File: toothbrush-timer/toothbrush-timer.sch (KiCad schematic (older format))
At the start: 19 parts, among them Q1 IRL2244, Q2 IRL6244, SW1 Power, U1 Arduino_Pro_Mini

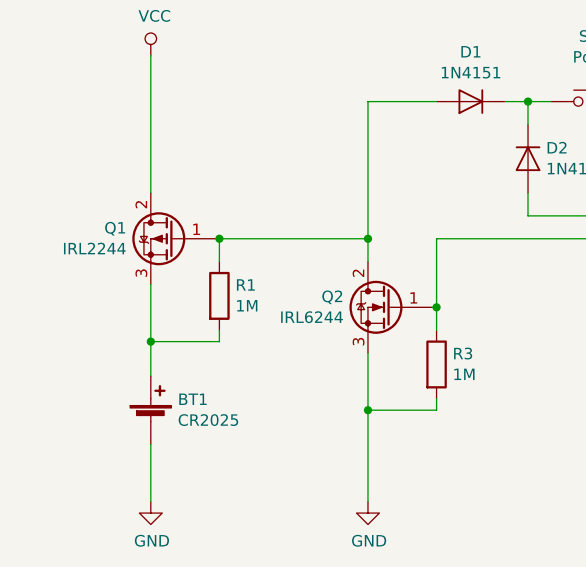
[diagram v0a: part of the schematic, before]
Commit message: Updated toohtbrush-timer
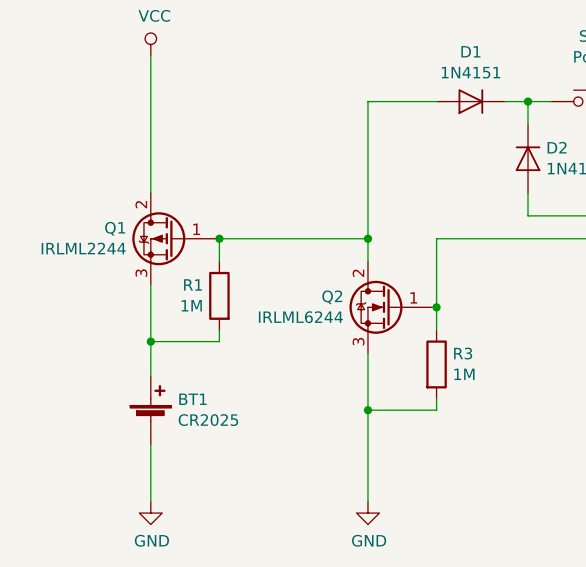
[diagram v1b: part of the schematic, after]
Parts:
- Q1: value IRL2244 -> IRLML2244
- Q2: value IRL6244 -> IRLML6244
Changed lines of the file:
@@
 F 3 "~" H 1350 2150 50  0001 C CNN
 	1    1350 2150
-	1    0    0    -1
+	-1   0    0    -1
 $EndComp
 $Comp
@@
 P 2100 2200
 F 0 "Q2" H 2306 2246 50  0000 L CNN
-F 1 "IRL6244" H 2306 2155 50  0000 L CNN
+F 1 "IRLML6244" H 2306 2155 50  0000 L CNN
 F 2 "" H 2300 2300 50  0001 C CNN
 F 3 "~" H 2100 2200 50  0001 C CNN
@@
 P 1150 1900
 F 0 "Q1" H 1356 1946 50  0000 L CNN
-F 1 "IRL2244" H 1356 1855 50  0000 L CNN
+F 1 "IRLML2244" H 1356 1855 50  0000 L CNN
 F 2 "" H 1350 2000 50  0001 C CNN
 F 3 "~" H 1150 1900 50  0001 C CNN
